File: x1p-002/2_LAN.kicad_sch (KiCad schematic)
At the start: 54 parts, among them U1 LAN9514, U5 AT93C66B-SSHM-T, X1 25MHz

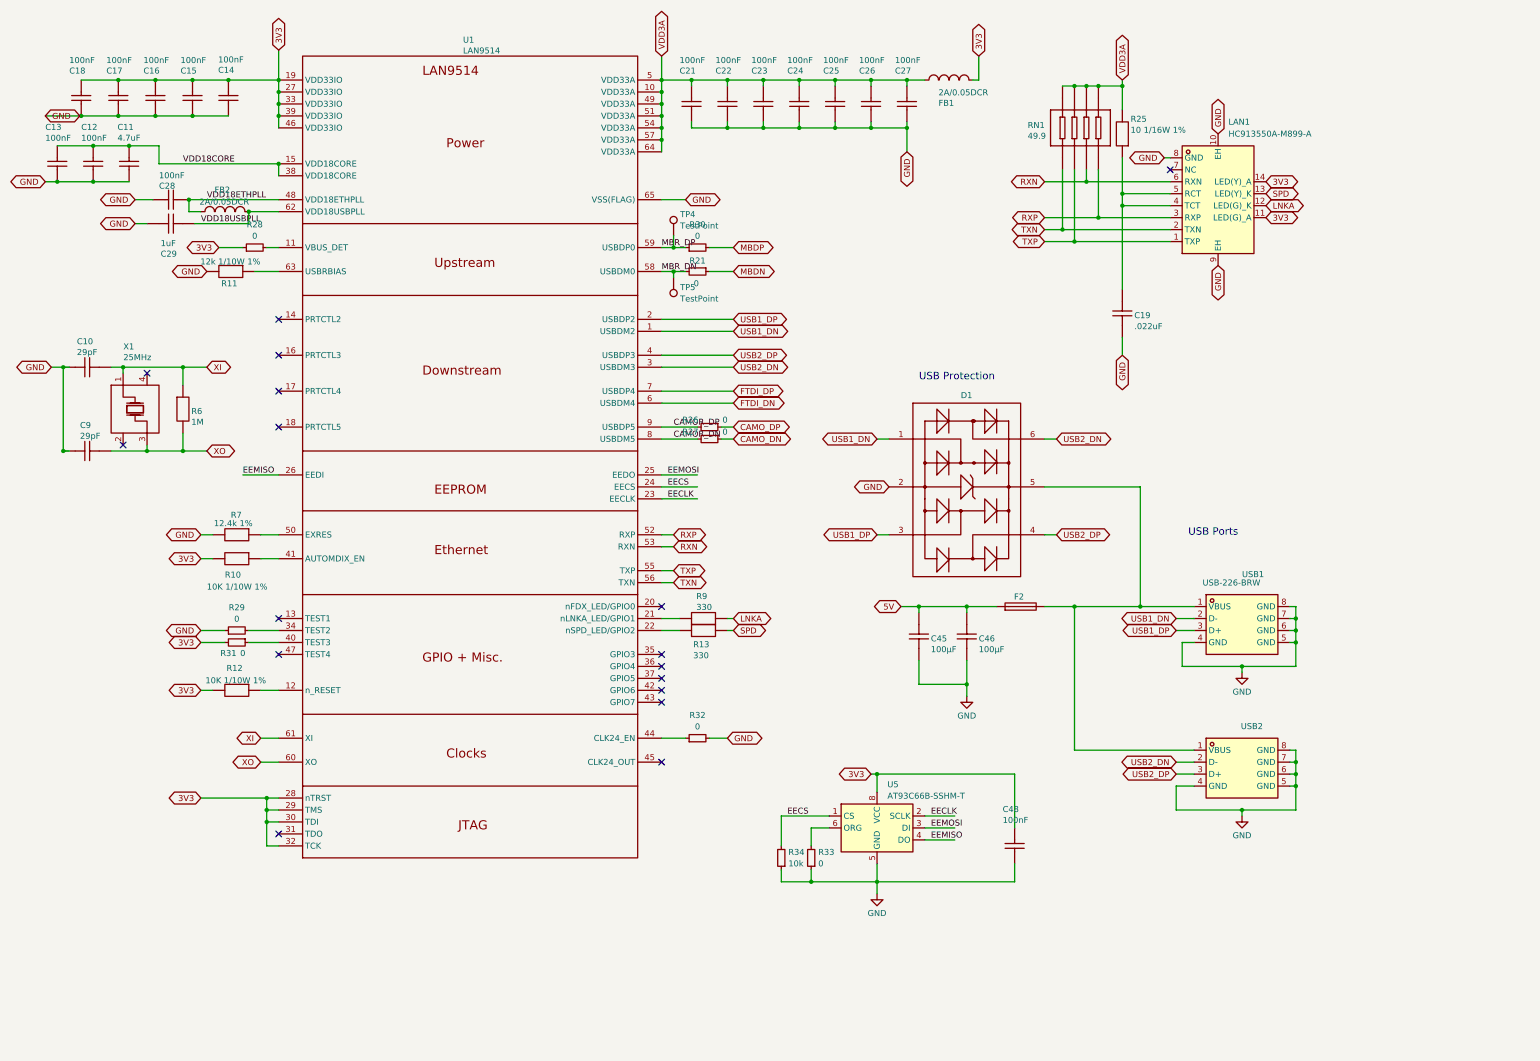
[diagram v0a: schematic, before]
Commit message: X1P-002: schematic: redesign with larger 5V buck (#60), add 3V3 buck (#63), add OCP circuits for 3V3 and 5V (but not connected to user ports yet; #61)
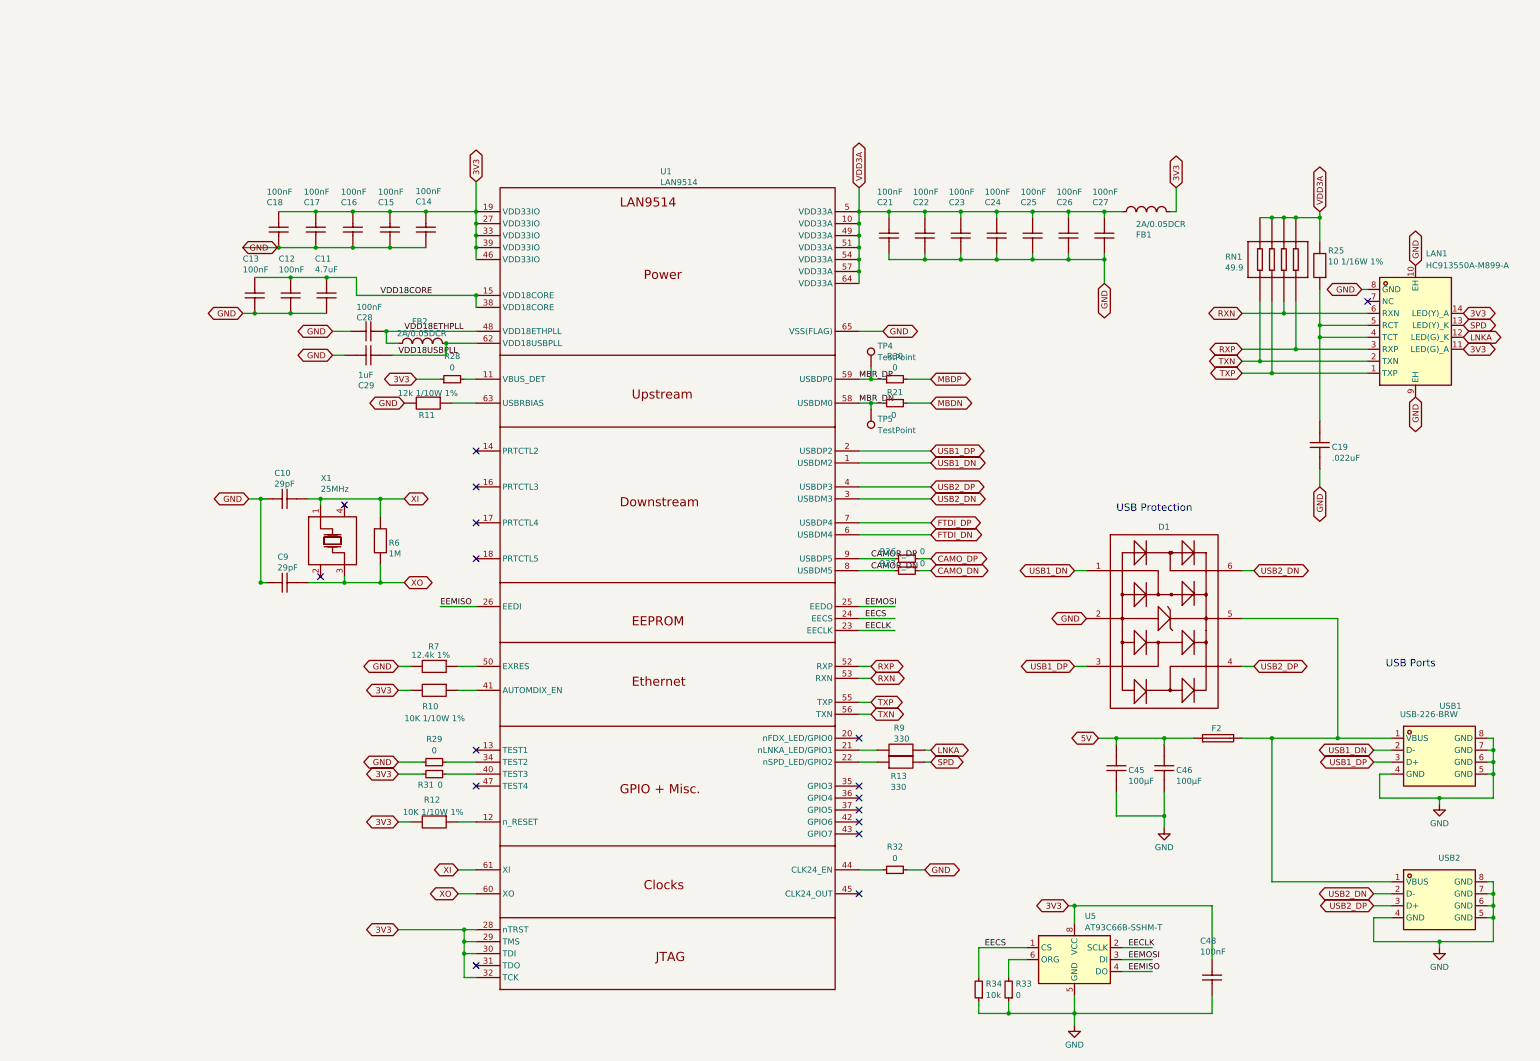
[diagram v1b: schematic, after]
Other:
- title: (none) -> X1Plus Expansion Board: X1P-002
- moved on the sheet: C10, C11, C12, C13, C14, C15, C16, C17, C18, C19, C21, C22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
